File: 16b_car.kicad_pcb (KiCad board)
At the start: 2 copper layers, 38 parts, among them J1 Conn_02x10_Odd_Even, J2 Conn_01x08_Female, J3 Conn_01x06_Female, J5 Conn_01x08_Female, J6 Conn_02x10_Odd_Even, M4 MountingHole_4.3mm_M4_DIN965_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, Q1 Q_NPN_BCE, Q2 Q_NPN_BCE, SW1 SW_DIP_x01, SW2 SW_DIP_x01, U1 LM6482IN/NOPB, U2 LM317T, U3 LM317T

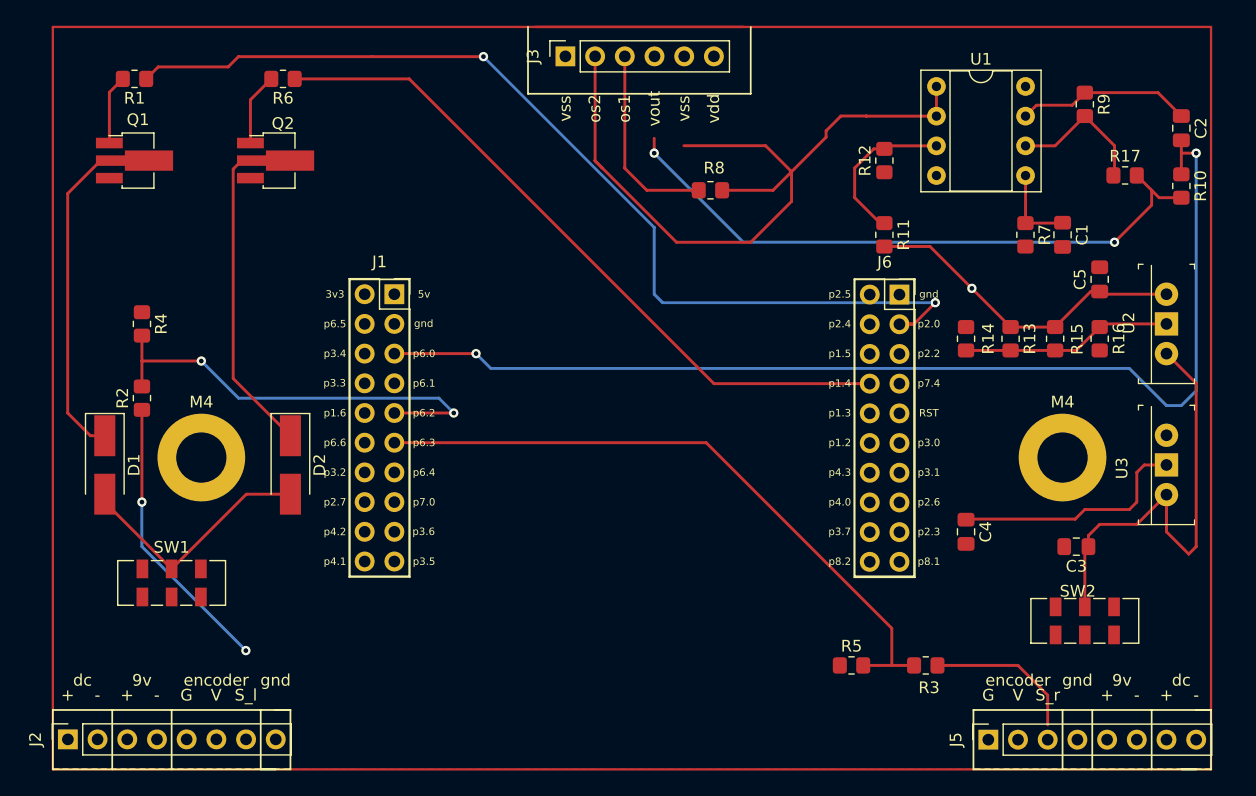
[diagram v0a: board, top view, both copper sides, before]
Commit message: 0 errors, 0 warnings
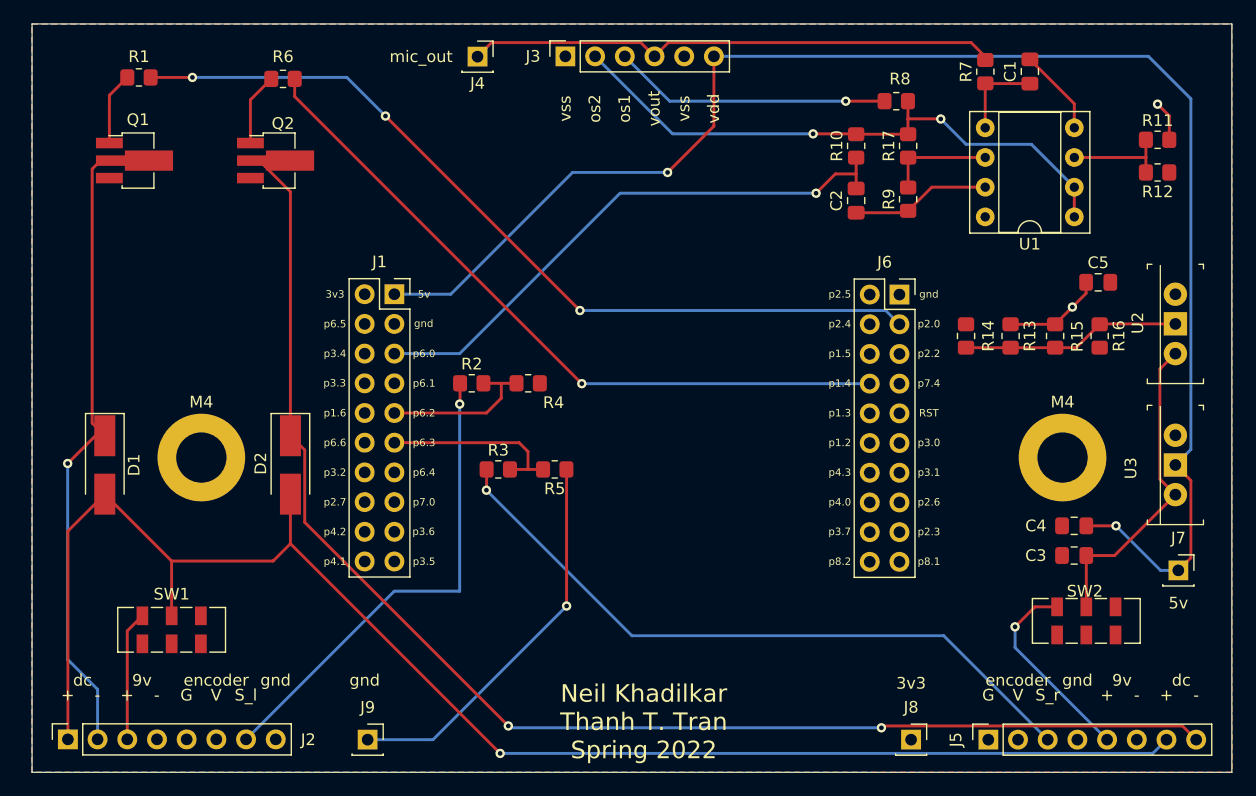
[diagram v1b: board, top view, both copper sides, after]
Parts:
- added J4: Conn_01x01_Female, Connector_PinSocket_2.54mm:PinSocket_1x01_P2.54mm_Vertical, F.Cu at (206.5, 94.0)
- added J7: Conn_01x01_Female, Connector_PinSocket_2.54mm:PinSocket_1x01_P2.54mm_Vertical, F.Cu at (266.4, 137.9)
- added J8: Conn_01x01_Female, Connector_PinSocket_2.54mm:PinSocket_1x01_P2.54mm_Vertical, F.Cu at (243.6, 152.4)
- added J9: Conn_01x01_Female, Connector_PinSocket_2.54mm:PinSocket_1x01_P2.54mm_Vertical, F.Cu at (197.1, 152.4)
- moved R3 40.2 mm to (208.3, 129.3), turned to 0 degrees
- moved R4 33.4 mm to (210.8, 121.9), turned to 180 degrees
- moved R5 30.4 mm to (213.1, 129.3), turned to 180 degrees
- moved C2 28.5 mm to (238.9, 106.3), turned to 90 degrees
- moved R2 28.2 mm to (206.0, 121.9), turned to 0 degrees
- moved R10 28.0 mm to (238.9, 101.6), turned to 90 degrees
- moved R11 24.7 mm to (264.7, 101.1), turned to 0 degrees
- moved R12 23.4 mm to (264.7, 103.9), turned to 180 degrees
- moved R17 18.7 mm to (243.3, 101.6), turned to 90 degrees
- moved R8 17.6 mm to (242.3, 97.8)
- moved R9 17.2 mm to (243.3, 106.2), turned to 90 degrees
- moved U1 16.2 mm to (257.5, 107.7), turned to 180 degrees
- moved R7 14.4 mm to (249.9, 95.3), turned to 90 degrees
- moved C1 14.2 mm to (253.7, 95.2), turned to 90 degrees
- moved C4 9.26 mm to (257.5, 134.1), turned to 180 degrees
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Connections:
- C1 pad 2: Gr -> GND
- C3 pad 2: Gr -> GND
- C4 pad 2: Gr -> GND
- C5 pad 1: Vl -> 3.3V
- C5 pad 2: Gr -> GND
- J1 pad 1: unconnected-(J1-Pad1) -> 5V
- J1 pad 3: unconnected-(J1-Pad3) -> GND
- J2 pad 4: 9v -l -> GND
- J2 pad 5: Gr -> GND
- J2 pad 6: Vl -> 3.3V
- J2 pad 7: P6.2 -> Sl
- J2 pad 8: gndl -> GND
- J3 pad 1: vss -> GND
- J3 pad 2: HALF RAIL -> HALF_RAIL
- J3 pad 4: vout -> MIC_OUT
- J3 pad 5: Vl -> GND
- J3 pad 6: vdd -> 5V
- J5 pad 1: Gr -> GND
- J5 pad 2: Vl -> 3.3V
- J5 pad 3: P6.3 -> Sr
- J5 pad 4: gndr -> GND
- J5 pad 6: 9v -r -> GND
- J6 pad 1: unconnected-(J6-Pad1) -> GND
- Q1 pad 3: Gr -> GND
- Q2 pad 3: Gr -> GND
- R11 pad 2: Vl -> 3.3V
- R12 pad 1: Gr -> GND
- R13 pad 1: Vl -> 3.3V
- R14 pad 2: Gr -> GND
- R15 pad 1: Vl -> 3.3V
- R16 pad 2: Gr -> GND
- R2 pad 1: Vl -> Sl
- R3 pad 1: SIGNAL_RIGHT -> Sr
- R4 pad 1: Gr -> GND
- R8 pad 2: HALF RAIL -> HALF_RAIL
- U1 pad 1: HALF RAIL -> HALF_RAIL
- U1 pad 2: HALF RAIL -> HALF_RAIL
- U1 pad 4: Gr -> GND
- U1 pad 8: Vl -> 3.3V
- U2 pad 3: Vl -> 3.3V
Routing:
- net 5V: track 20.6 -> 132.9 mm, vias 0 -> 2
- net dc +l: track 21.6 -> 132.9 mm, vias 0 -> 1
- net dc -r: track 26.7 -> 117.3 mm, vias 0 -> 2
- net HALF RAIL: track 67.5 -> 0.00 mm
- net Sr: track 0.00 -> 58.6 mm, vias 0 -> 1
- net Vl: track 52.6 -> 0.00 mm, vias 3 -> 0
- net P6.0: track 95.4 -> 48.5 mm, vias 2 -> 1
- net MIC_OUT: track 0.00 -> 45.7 mm
- net Sl: track 0.00 -> 41.3 mm, vias 0 -> 1
- net GND: track 0.00 -> 40.9 mm, vias 0 -> 1
- net P6.3: track 56.6 -> 16.1 mm
- net dc -l: track 27.6 -> 53.9 mm, vias 0 -> 1
- net P6.2: track 37.9 -> 13.8 mm, vias 2 -> 0
- net 9v +r: track 0.00 -> 17.2 mm, vias 0 -> 1
- net SIGNAL_RIGHT: track 13.0 -> 0.00 mm
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- added copper zone on B.Cu, net 3.3V
- added copper zone on F.Cu, net GND
- removed copper zone on F.Cu, net Gr
- removed copper zone on B.Cu, net Vl
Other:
- board outline added: 102.6 x 64 mm
- board text added: "Neil Khadilkar Thanh T. Tran Spring 2022"
- board text added: "mic_out"
